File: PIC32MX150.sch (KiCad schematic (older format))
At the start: 39 parts, among them J1 GPIO_1, J2 USB_B_Micro, J3 Barrel_Jack, J4 ICSP, J5 GPIO_2, SW1 RST, SW2 SW_SPDT, U1 PIC32MX150F128D-IPT, U2 LM22676MR-ADJ, U3 CH340C, Y1 TSX3225

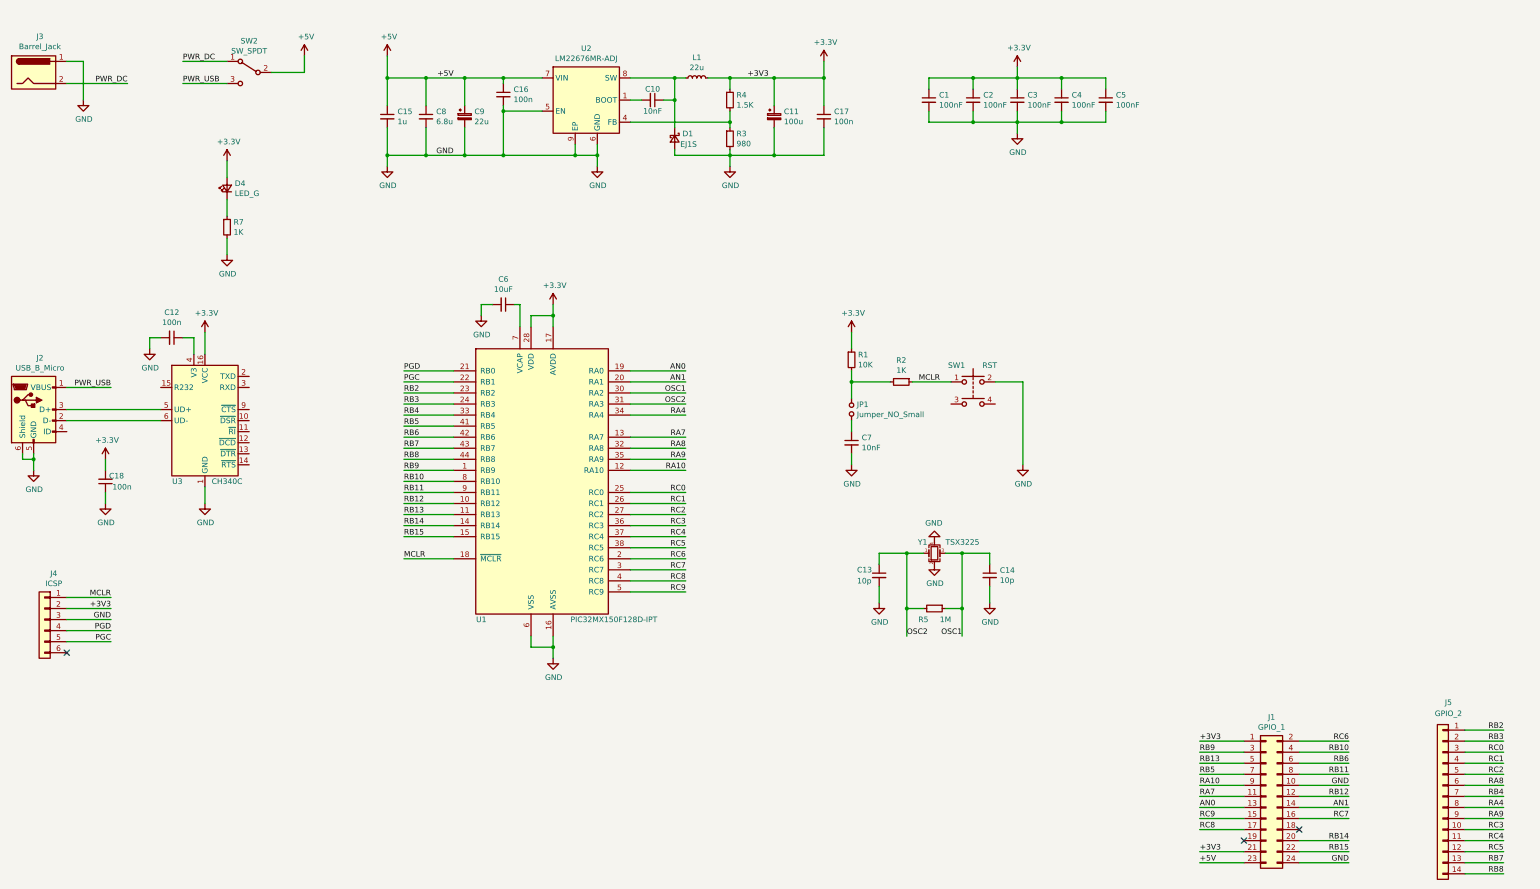
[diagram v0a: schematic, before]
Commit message: gerber
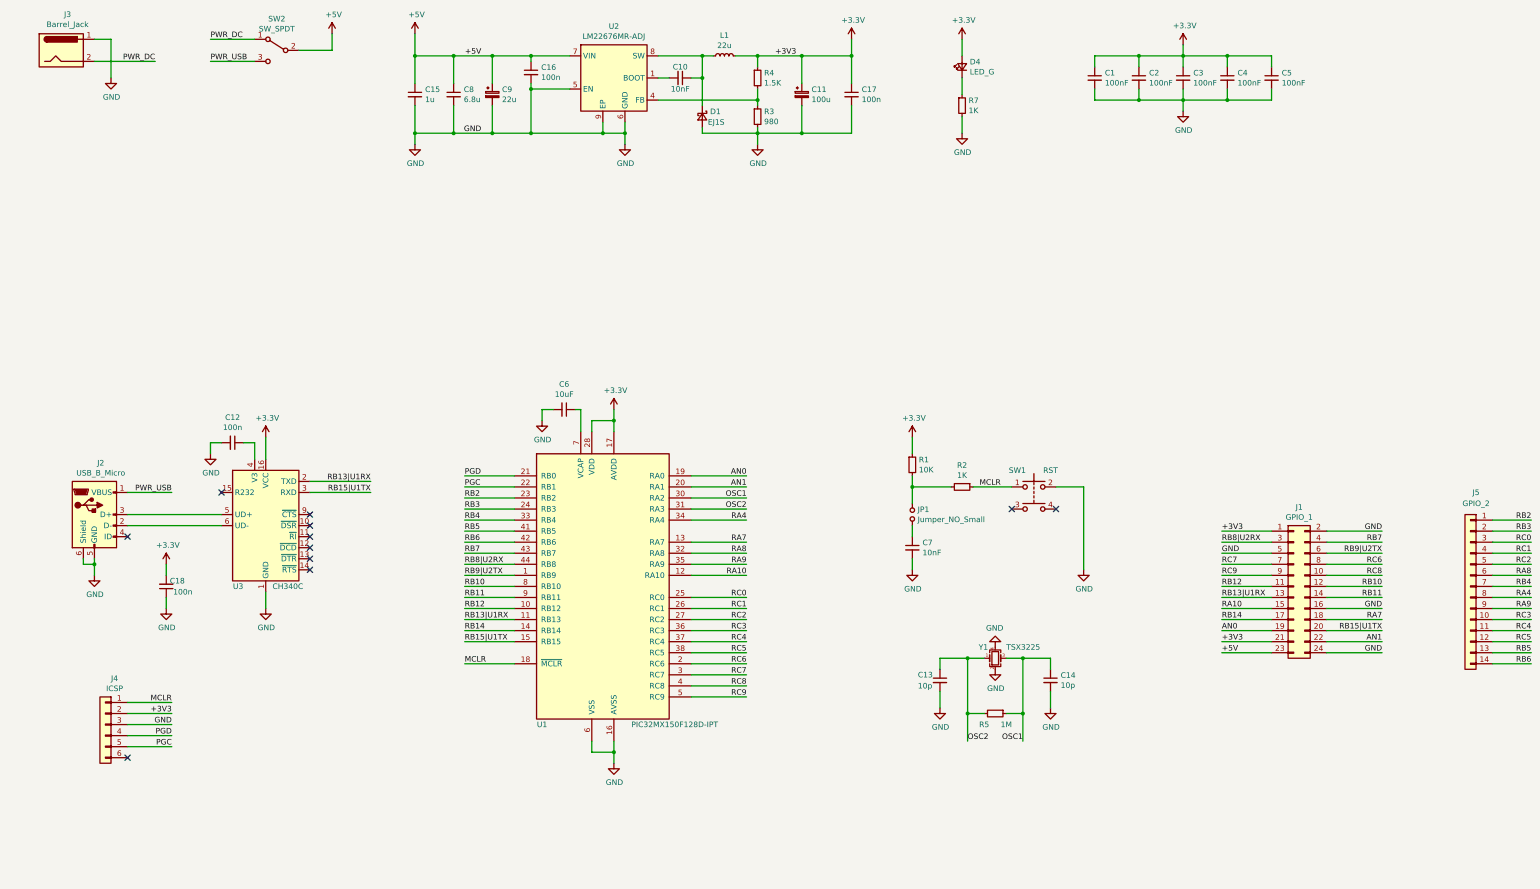
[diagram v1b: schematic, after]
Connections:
- net AN0: now also J1.19 (Pin_19); no longer J1.13 (Pin_13)
- net AN1: now also J1.22 (Pin_22); no longer J1.14 (Pin_14)
- net GND: now also J1.16 (Pin_16), J1.2 (Pin_2), J1.5 (Pin_5); no longer J1.10 (Pin_10)
- net RA10: now also J1.15 (Pin_15); no longer J1.9 (Pin_9)
- net RA7: now also J1.18 (Pin_18); no longer J1.11 (Pin_11)
- net RB10: now also J1.12 (Pin_12); no longer J1.4 (Pin_4)
- net RB11: now also J1.14 (Pin_14); no longer J1.8 (Pin_8)
- net RB12: now also J1.11 (Pin_11); no longer J1.12 (Pin_12)
- net RB14: now also J1.17 (Pin_17); no longer J1.20 (Pin_20)
- net RB5: now also J5.13 (Pin_13); no longer J1.7 (Pin_7)
- net RB6: now also J5.14 (Pin_14); no longer J1.6 (Pin_6)
- net RB7: now also J1.4 (Pin_4); no longer J5.13 (Pin_13)
- net RC6: now also J1.8 (Pin_8); no longer J1.2 (Pin_2)
- net RC7: now also J1.7 (Pin_7); no longer J1.16 (Pin_16)
- net RC8: now also J1.10 (Pin_10); no longer J1.17 (Pin_17)
- net RC9: now also J1.9 (Pin_9); no longer J1.15 (Pin_15)
- net RB13|U1RX: now reaches U3.2 (TXD)
- net RB13|U1RX: now also J1.13 (Pin_13), U1.11 (RB13)
- net RB15|U1TX: now reaches U3.3 (RXD)
- net RB15|U1TX: now also J1.20 (Pin_20), U1.15 (RB15)
- removed net RB13: J1.5 (Pin_5), U1.11 (RB13)
- removed net RB15: J1.22 (Pin_22), U1.15 (RB15)
- net RB8 renamed RB8|U2RX
- net RB8|U2RX: now also J1.3 (Pin_3); no longer J5.14 (Pin_14)
- net RB9 renamed RB9|U2TX
- net RB9|U2TX: now also J1.6 (Pin_6); no longer J1.3 (Pin_3)
- no-connect marks 3 -> 11
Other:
- moved on the sheet: C1, C10, C11, C12, C13, C14, C15, C16, C17, C18, C2, C3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
